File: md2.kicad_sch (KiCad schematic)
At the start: 44 parts, among them IC1 TC74HC4066AP_F_, IC2 TC74HC4066AP_F_, IC3 TC74HC04AP, IC4 TB6643KQ, IC5 TB6643KQ, IC6 TB6643KQ, IC7 TB6643KQ, J1 Conn_01x02_Pin, J10 Conn_01x02_Pin, J3 Conn_02x13_Odd_Even, J5 XT30PW-M, J6 XT30PW-M, J7 XT30PW-M, J8 XT30PW-M, J9 Conn_01x02_Pin, SW1 SW_Push, SW2 SW_Push, SW3 SW_Push, SW4 SW_Push, SW5 SW_Push, SW6 SW_Push, SW7 SW_Push, SW8 SW_Push, SW9 SW_Push, U1 NJM7805FA, U2 SeeeduinoXIAO

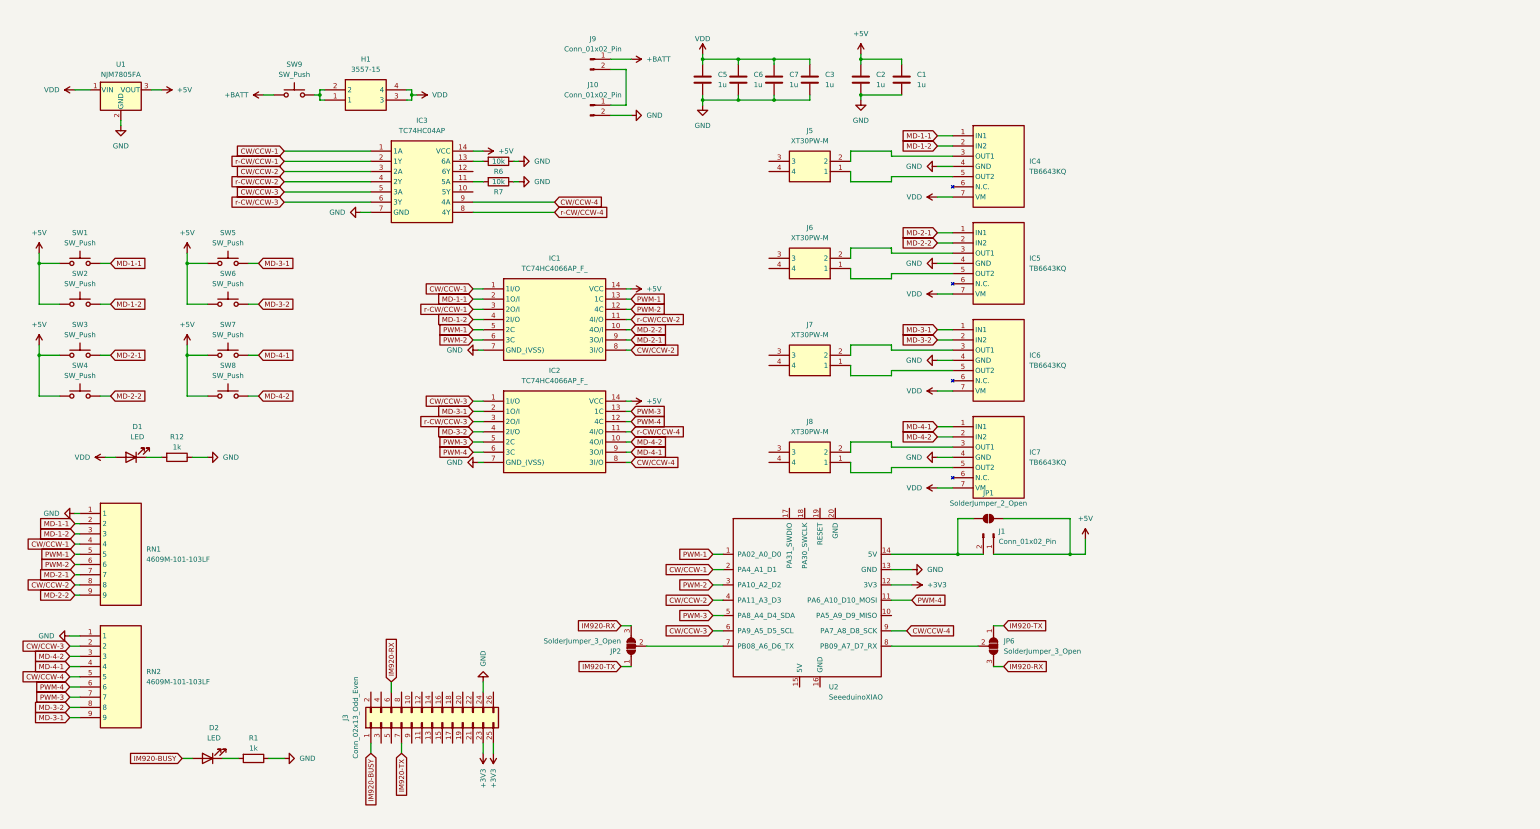
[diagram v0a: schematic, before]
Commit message: update
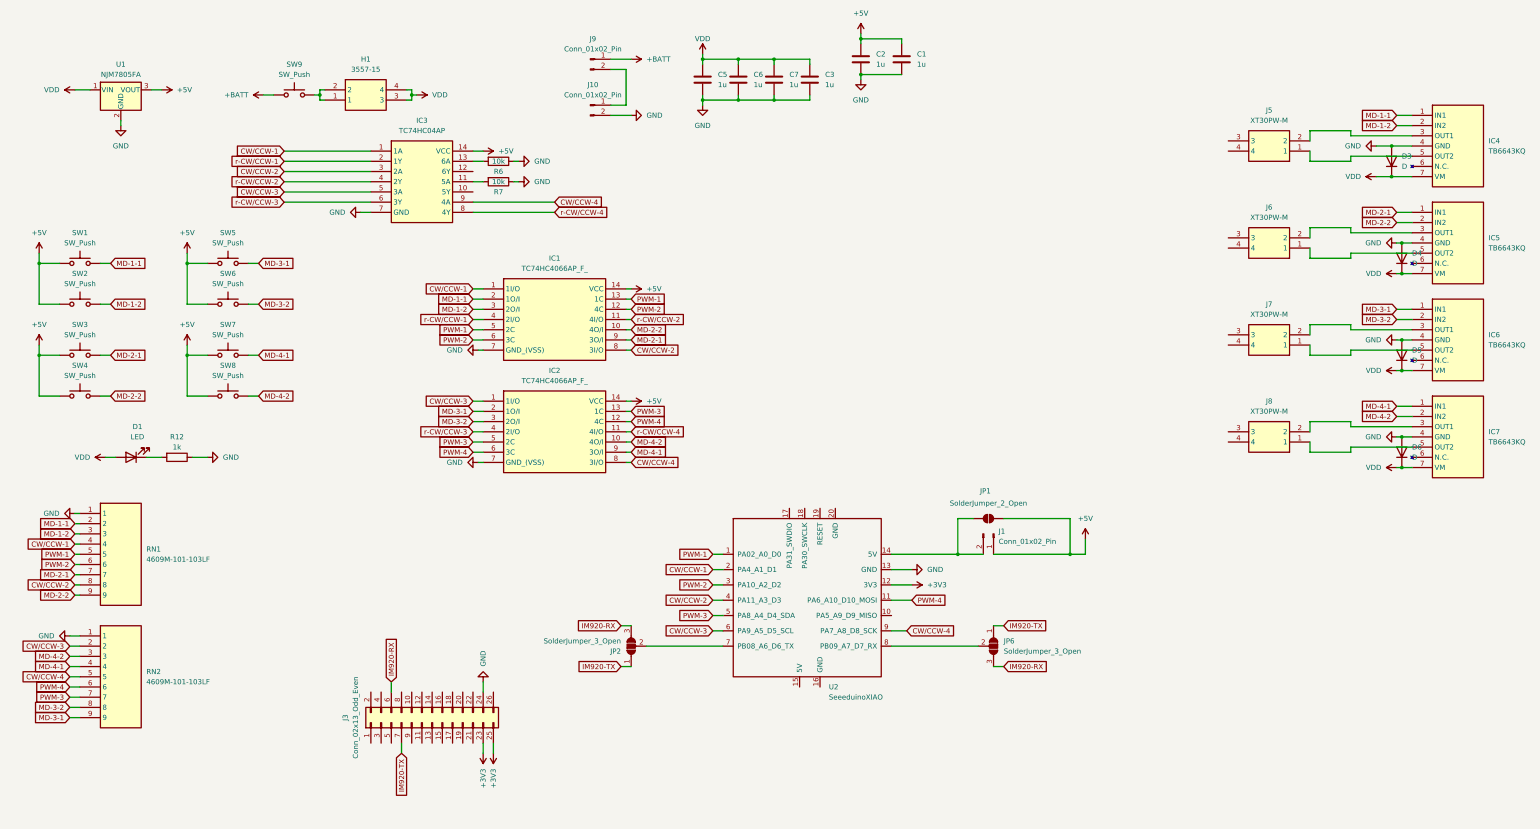
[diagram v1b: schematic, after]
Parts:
- removed D2: LED, LED_THT:LED_D3.0mm, symbol Device:LED
- removed R1: 1k, Resistor_THT:R_Axial_DIN0207_L6.3mm_D2.5mm_P10.16mm_Horizontal, symbol Device:R
- added D3, D4, D5, D6: D, Diode_THT:D_DO-41_SOD81_P10.16mm_Horizontal, symbol Device:D
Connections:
- net GND: now also D3.2 (A), D4.2 (A), D5.2 (A), D6.2 (A)
- net MD-1-2: now also IC1.3 (2O/I); no longer IC1.4 (2I/O)
- net MD-3-2: now also IC2.3 (2O/I); no longer IC2.4 (2I/O)
- net VDD: now also D3.1 (K), D4.1 (K), D5.1 (K), D6.1 (K)
- net r-CW/CCW-1: now also IC1.4 (2I/O); no longer IC1.3 (2O/I)
- net r-CW/CCW-3: now also IC2.4 (2I/O); no longer IC2.3 (2O/I)
- net IM920-BUSY: no longer names the net of J3.1 (Pin_1)
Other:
- moved on the sheet: C1, C2, IC4, IC5, IC6, IC7, J5, J6, J7, J8
